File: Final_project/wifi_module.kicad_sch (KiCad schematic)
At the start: 12 parts, among them U4 ESP32-WROOM-32

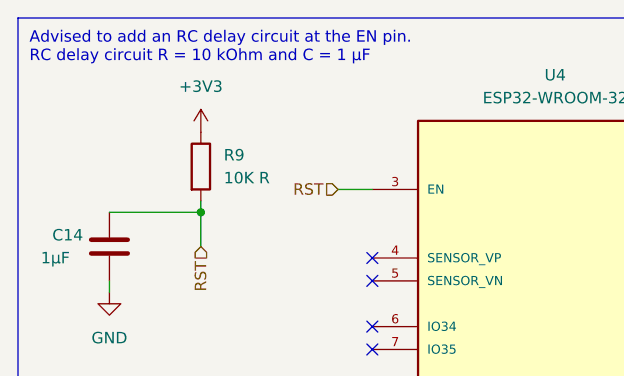
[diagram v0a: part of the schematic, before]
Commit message: almost finished layout
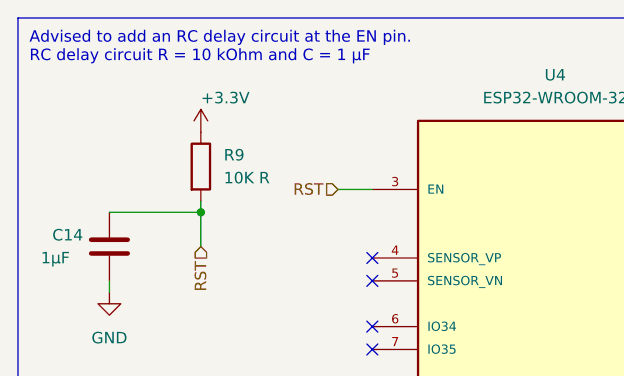
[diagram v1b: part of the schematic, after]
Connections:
- net +3V3: no longer R9.1
- new net +3.3V: R9.1
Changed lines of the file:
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@@
     (effects (font (size 1.27 1.27)) (justify right))
+  )
+  (symbol (lib_id "power:+3.3V") (at 35.56 26.67 0) (unit 1)
+    (in_bom yes) (on_board yes)
+    (property "Reference" "#PWR0136" (id 0) (at 35.56 30.48 0)
+      (effects (font (size 1.27 1.27)) hide)
+    )
+    (property "Value" "+3.3V" (id 1) (at 35.5601 22.86 0)
+      (effects (font (size 1.27 1.27)) (justify left))
+    )
+    (property "Footprint" "" (id 2) (at 35.56 26.67 0)
+      (effects (font (size 1.27 1.27)) hide)
+    )
+    (property "Datasheet" "" (id 3) (at 35.56 26.67 0)
+      (effects (font (size 1.27 1.27)) hide)
+    )
+    (pin "1")
   )
   (symbol (lib_id "ESP32-WROOM-32:ESP32-WROOM-32") (at 74.93 60.96 0) (unit 1)
@@
       (effects (font (size 1.27 1.27)) hide)
     )
-    (pin "1")
-  )
-  (symbol (lib_id "power:+3V3") (at 35.56 26.67 0) (unit 1)
-    (in_bom yes) (on_board yes) (fields_autoplaced)
-    (property "Reference" "#PWR0136" (id 0) (at 35.56 30.48 0)
-      (effects (font (size 1.27 1.27)) hide)
-    )
-    (property "Value" "+3V3" (id 1) (at 35.56 21.59 0))
-    (property "Footprint" "" (id 2) (at 35.56 26.67 0)
-      (effects (font (size 1.27 1.27)) hide)
-    )
-    (property "Datasheet" "" (id 3) (at 35.56 26.67 0)
-      (effects (font (size 1.27 1.27)) hide)
-    )
